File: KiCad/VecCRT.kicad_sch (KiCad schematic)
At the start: 80 parts, among them J1 RaspiGPIO, J2 K2, J3 Conn_01x03, J4 Conn_01x06, J5 Conn_01x03, J6 Conn_01x06, J7 K2, Q1 2N7000, Q10 2N7000, Q2 2N7002, Q3 2N7002, Q4 2N7000, Q5 2N7002, Q6 2N7002, Q9 2N7000, U1 MCP4822, U2 4066, U3 4066, U4 TL072, U5 TL072, U6 4011, U7 40106, U8 4011

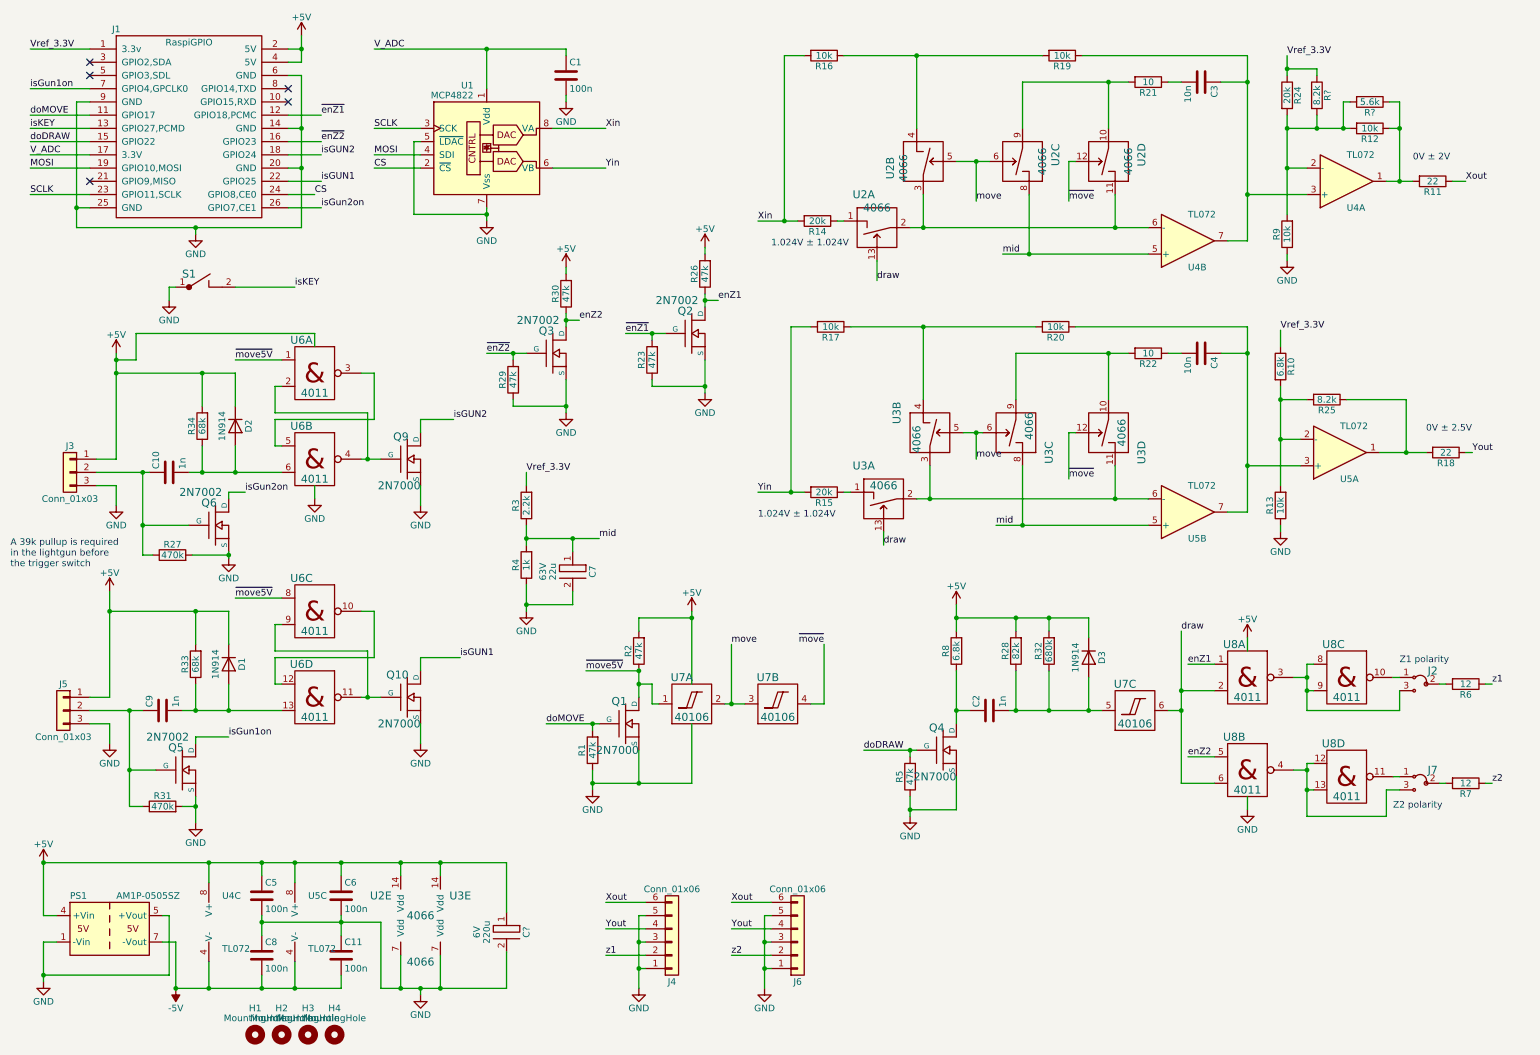
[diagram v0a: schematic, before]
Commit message: before 1.0
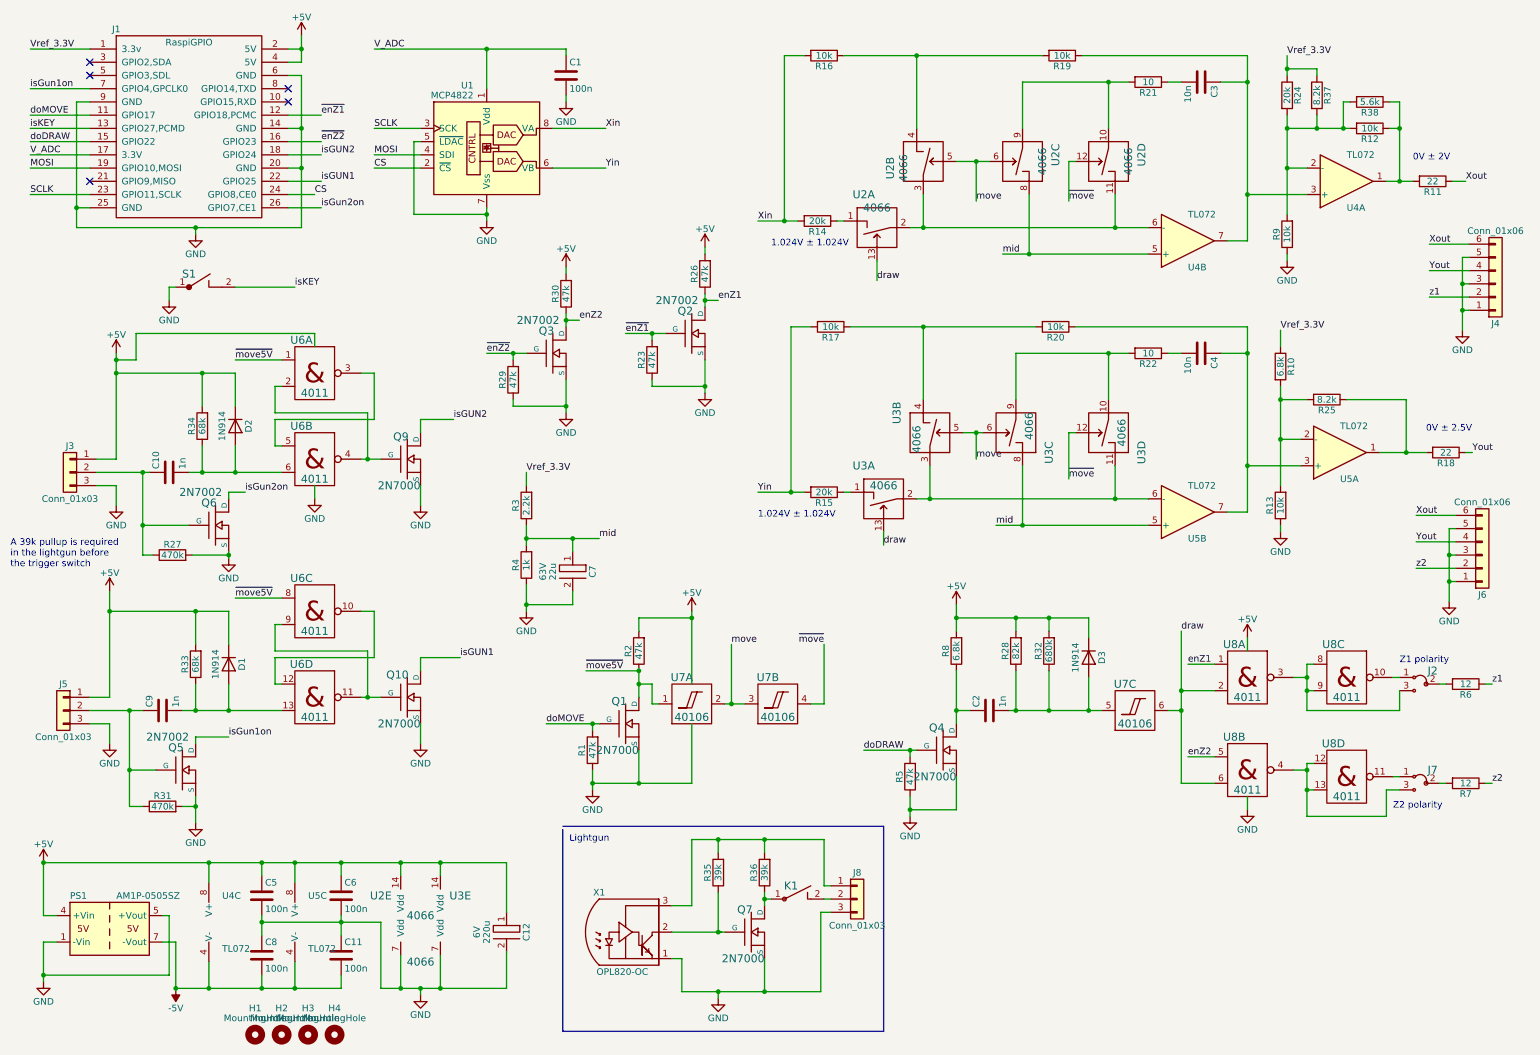
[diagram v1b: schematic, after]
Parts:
- added J8: Conn_01x03, RG:PSS_3, symbol Connector_Generic:Conn_01x03
- added K1: SchEin, PINHEAD1-2, symbol rg:SchEin
- added Q7: 2N7000, RG:FETsgd_inline, symbol rg:BS170
- added R35, R36: 39k, RG:R4-2, symbol Device:R
- added X1: OPL820-OC, symbol rg:OPL820-OC
- gave numbers to parts that had none: 3
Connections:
- net GND: now also J8.3 (Pin_3), Q7.S, X1.1
- new net: K1.1, Q7.D, R36.1
- new net: J8.2 (Pin_2), K1.2
- new net: Q7.G, R35.1, X1.2
- new net: J8.1 (Pin_1), R35.2, R36.2, X1.3
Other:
- note added: "Lightgun"
- moved on the sheet: J4, J6
